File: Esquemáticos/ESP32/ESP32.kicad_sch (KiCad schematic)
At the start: 1 part

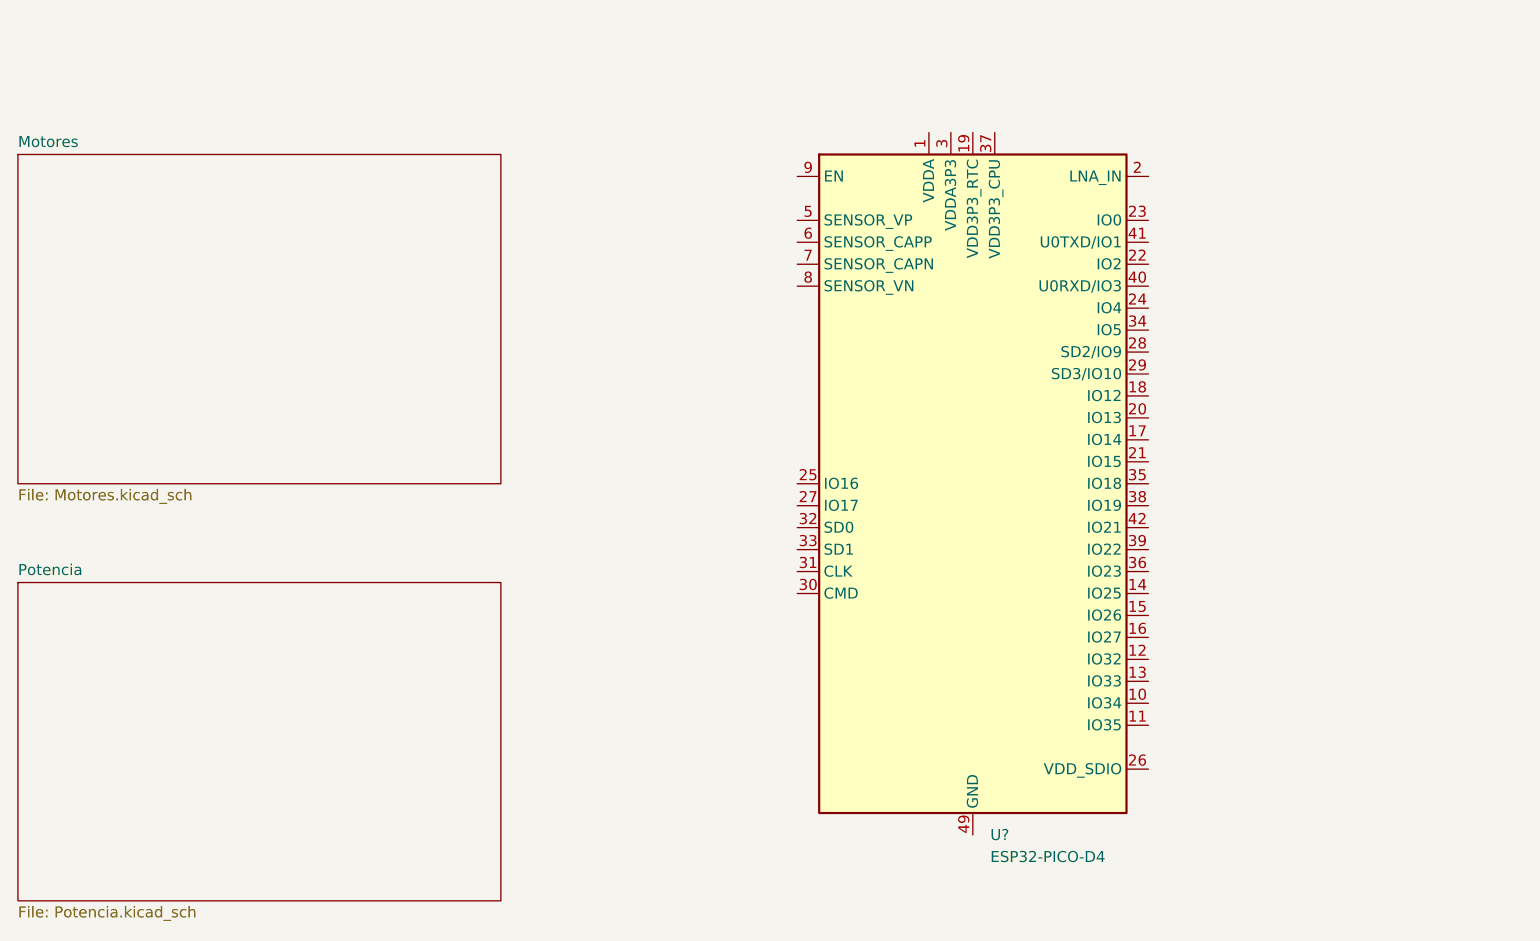
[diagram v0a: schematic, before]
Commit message: mensaje
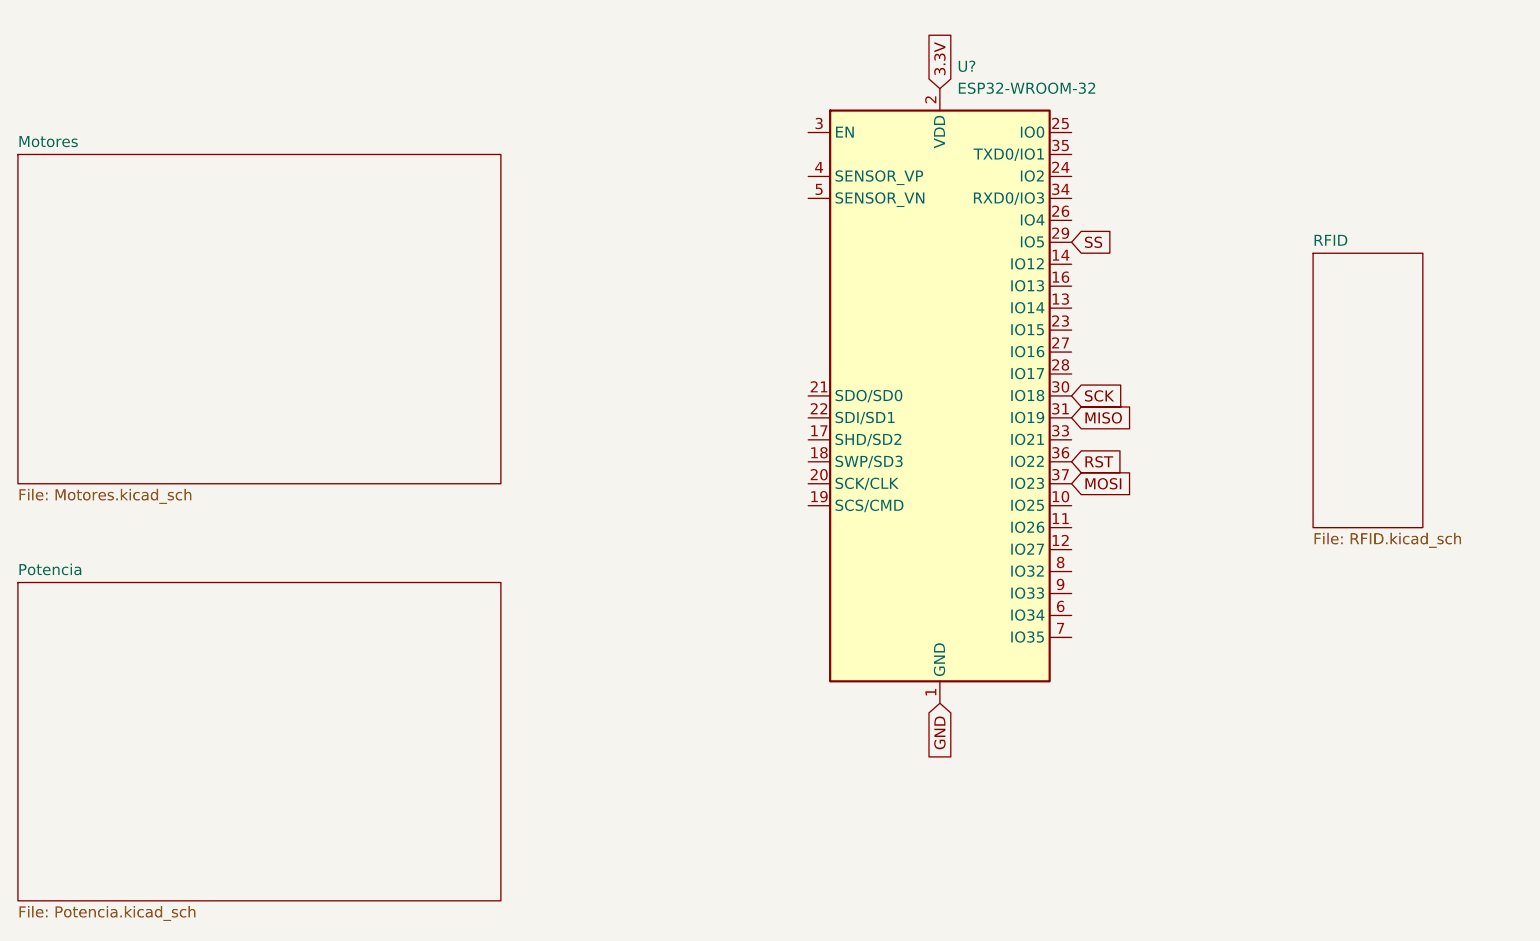
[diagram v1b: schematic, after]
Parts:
- removed U?: ESP32-PICO-D4, Package_DFN_QFN:QFN-48-1EP_7x7mm_P0.5mm_EP5.3x5.3mm, symbol RF_Module:ESP32-PICO-D4
- added U?: ESP32-WROOM-32, RF_Module:ESP32-WROOM-32, symbol RF_Module:ESP32-WROOM-32
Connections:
- new net 3.3V: U?.2 (VDD)
- new net GND: U?.1 (GND), U?.15 (GND), U?.38 (GND), U?.39 (GND)
- new net MISO: U?.31 (IO19)
- new net MOSI: U?.37 (IO23)
- new net RST: U?.36 (IO22)
- new net SCK: U?.30 (IO18)
- new net SS: U?.29 (IO5)
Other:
- added sheet RFID (RFID.kicad_sch)
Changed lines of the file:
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@@
 (kicad_sch (version 20211123) (generator eeschema)
   (paper "A4")
-  (symbol (lib_id "RF_Module:ESP32-PICO-D4") (at 144.78 100.33 0) (unit 1)
+  (global_label "GND" (shape input) (at 140.97 125.73 270) (fields_autoplaced)
+    (effects (font (size 1.27 1.27)) (justify right))
+    (property "Referencias entre hojas" "${INTERSHEET_REFS}" (id 0) (at 140.8906 132.0136 90)
+      (effects (font (size 1.27 1.27)) (justify right) hide)
+    )
+  )
+  (global_label "3.3V" (shape input) (at 140.97 54.61 90) (fields_autoplaced)
+    (effects (font (size 1.27 1.27)) (justify left))
+    (property "Referencias entre hojas" "${INTERSHEET_REFS}" (id 0) (at 140.8906 48.0845 90)
+      (effects (font (size 1.27 1.27)) (justify left) hide)
+    )
+  )
+  (global_label "MISO" (shape input) (at 156.21 92.71 0) (fields_autoplaced)
+    (effects (font (size 1.27 1.27)) (justify left))
+    (property "Referencias entre hojas" "${INTERSHEET_REFS}" (id 0) (at 163.2193 92.6306 0)
+      (effects (font (size 1.27 1.27)) (justify left) hide)
+    )
+  )
+  (global_label "SCK" (shape input) (at 156.21 90.17 0) (fields_autoplaced)
+    (effects (font (size 1.27 1.27)) (justify left))
+    (property "Referencias entre hojas" "${INTERSHEET_REFS}" (id 0) (at 162.3726 90.0906 0)
+      (effects (font (size 1.27 1.27)) (justify left) hide)
+    )
+  )
+  (global_label "RST" (shape input) (at 156.21 97.79 0) (fields_autoplaced)
+    (effects (font (size 1.27 1.27)) (justify left))
+    (property "Referencias entre hojas" "${INTERSHEET_REFS}" (id 0) (at 162.0702 97.7106 0)
+      (effects (font (size 1.27 1.27)) (justify left) hide)
+    )
+  )
+  (global_label "SS" (shape input) (at 156.21 72.39 0) (fields_autoplaced)
+    (effects (font (size 1.27 1.27)) (justify left))
+    (property "Referencias entre hojas" "${INTERSHEET_REFS}" (id 0) (at 161.0421 72.3106 0)
+      (effects (font (size 1.27 1.27)) (justify left) hide)
+    )
+  )
+  (global_label "MOSI" (shape input) (at 156.21 100.33 0) (fields_autoplaced)
+    (effects (font (size 1.27 1.27)) (justify left))
+    (property "Referencias entre hojas" "${INTERSHEET_REFS}" (id 0) (at 163.2193 100.2506 0)
+      (effects (font (size 1.27 1.27)) (justify left) hide)
+    )
+  )
+  (symbol (lib_id "RF_Module:ESP32-WROOM-32") (at 140.97 90.17 0) (unit 1)
     (in_bom yes) (on_board yes) (fields_autoplaced)
-    (property "Reference" "U?" (id 0) (at 146.7994 140.97 0)
+    (property "Reference" "U?" (id 0) (at 142.9894 52.07 0)
       (effects (font (size 1.27 1.27)) (justify left))
     )
-    (property "Value" "ESP32-PICO-D4" (id 1) (at 146.7994 143.51 0)
+    (property "Value" "ESP32-WROOM-32" (id 1) (at 142.9894 54.61 0)
       (effects (font (size 1.27 1.27)) (justify left))
     )
-    (property "Footprint" "Package_DFN_QFN:QFN-48-1EP_7x7mm_P0.5mm_EP5.3x5.3mm" (id 2) (at 144.78 143.51 0)
+    (property "Footprint" "RF_Module:ESP32-WROOM-32" (id 2) (at 140.97 128.27 0)
       (effects (font (size 1.27 1.27)) hide)
     )
-    (property "Datasheet" "https://www.espressif.com/sites/default/files/documentation/esp32-pico-d4_datasheet_en.pdf" (id 3) (at 151.13 125.73 0)
+    (property "Datasheet" "https://www.espressif.com/sites/default/files/documentation/esp32-wroom-32_datasheet_en.pdf" (id 3) (at 133.35 88.9 0)
       (effects (font (size 1.27 1.27)) hide)
     )
@@
     (pin "39")
     (pin "4")
-    (pin "40")
-    (pin "41")
-    (pin "42")
-    (pin "43")
-    (pin "44")
-    (pin "45")
-    (pin "46")
-    (pin "47")
-    (pin "48")
-    (pin "49")
     (pin "5")
     (pin "6")
@@
     )
   )
+  (sheet (at 184.15 73.66) (size 12.7 31.75) (fields_autoplaced)
+    (stroke (width 0.1524) (type solid) (color 0 0 0 0))
+    (fill (color 0 0 0 0.0000))
+    (property "Sheet name" "RFID" (id 0) (at 184.15 72.9484 0)
+      (effects (font (size 1.27 1.27)) (justify left bottom))
+    )
+    (property "Sheet file" "RFID.kicad_sch" (id 1) (at 184.15 105.9946 0)
+      (effects (font (size 1.27 1.27)) (justify left top))
+    )
+  )
   (sheet (at 34.29 62.23) (size 55.88 38.1) (fields_autoplaced)
     (stroke (width 0.1524) (type solid) (color 0 0 0 0))
@@
     (path "/3dc66758-7067-4285-a03f-e9474bf12d83" (page "2"))
     (path "/e1e74fdb-71e2-41d9-bc36-66c7a8ec4b6a" (page "3"))
+    (path "/80dbd6db-b9cc-42d5-a40e-8d2c99f93a1b" (page "4"))
   )
   (symbol_instances
@@
       (reference "J2") (unit 1) (value "Conector para bobinas del motor 2") (footprint "")
     )
+    (path "/80dbd6db-b9cc-42d5-a40e-8d2c99f93a1b/3471c47f-a636-4058-83f1-2e9cb217714f"
+      (reference "J?") (unit 1) (value "Conn_RFID_SPI") (footprint "")
+    )
     (path "/3dc66758-7067-4285-a03f-e9474bf12d83/e33de0b8-310e-4c90-a1cc-6d9bb1ac1b41"
       (reference "J?") (unit 1) (value "Barrel_Jack") (footprint "")
@@
       (reference "U2") (unit 1) (value "ULN2003A") (footprint "")
     )
-    (path "/266e158e-7474-4de0-b2cb-c3efc5bc9c58"
-      (reference "U?") (unit 1) (value "ESP32-PICO-D4") (footprint "Package_DFN_QFN:QFN-48-1EP_7x7mm_P0.5mm_EP5.3x5.3mm")
-    )
     (path "/3dc66758-7067-4285-a03f-e9474bf12d83/43b937ef-b7e6-4e46-9361-ca0038217fbd"
       (reference "U?") (unit 1) (value "AMS1117-3.3") (footprint "Package_TO_SOT_SMD:SOT-223-3_TabPin2")
     )
+    (path "/7126fc01-b23f-49c1-b635-013e178bb3de"
+      (reference "U?") (unit 1) (value "ESP32-WROOM-32") (footprint "RF_Module:ESP32-WROOM-32")
+    )
     (path "/e1e74fdb-71e2-41d9-bc36-66c7a8ec4b6a/f7965755-6f1a-4b02-9c6c-4500de9fac77"
